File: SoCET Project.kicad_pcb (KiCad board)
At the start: 2 copper layers, 80.5 x 48.7 mm, 45 parts, among them J1 USB_C_Receptacle_USB2.0, J2 Conn_01x16_Female, J3 Conn_01x16_Female, J6 ICSP, SW1 SW_Push, U1 ATmega328P-A, U2 LM1117DT-ADJ, U3 FT232RL, Y1 16MHz

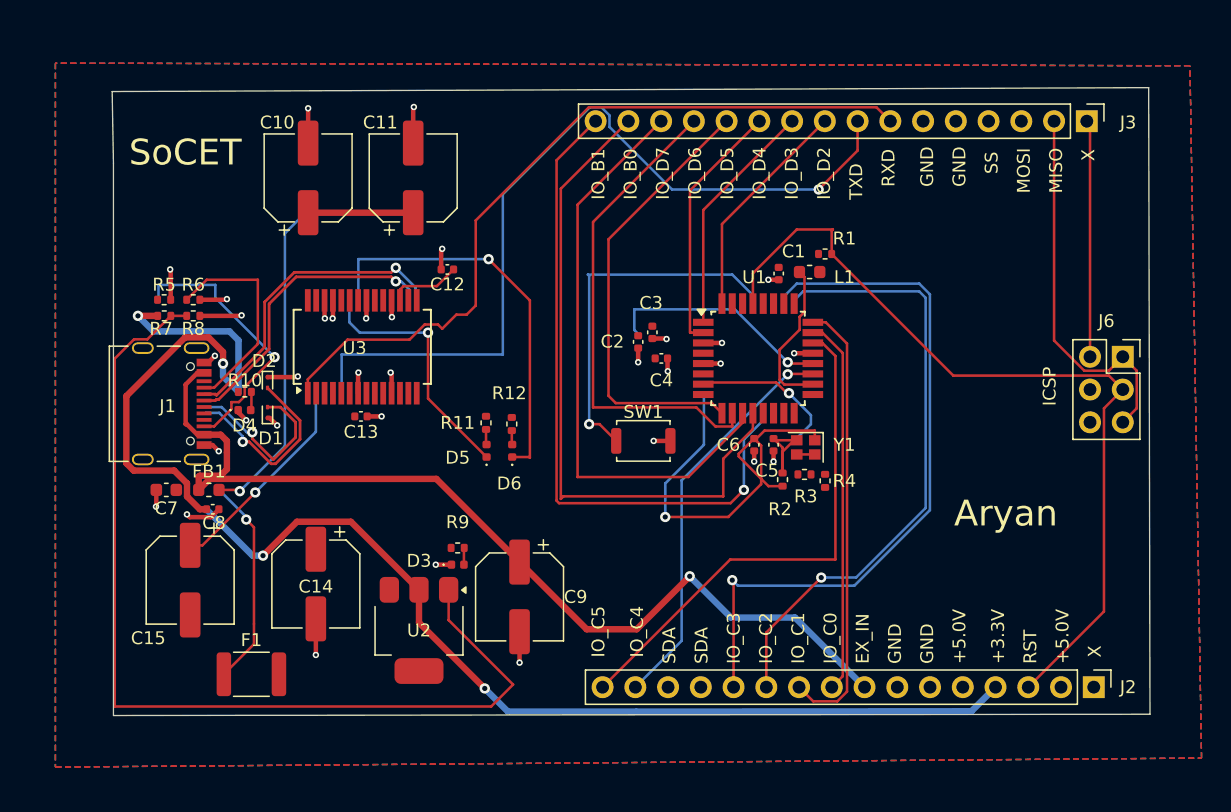
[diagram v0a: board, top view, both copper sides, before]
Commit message: Add files via upload
Completed SCH and DSG
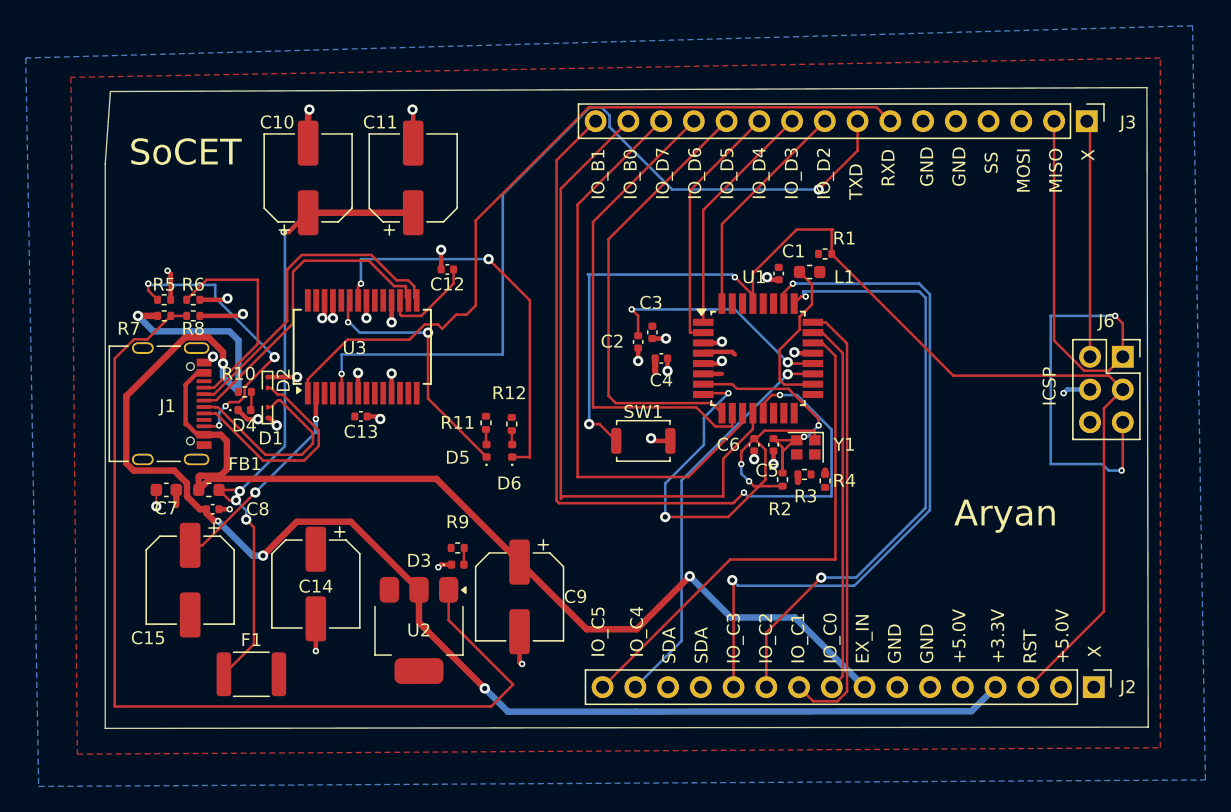
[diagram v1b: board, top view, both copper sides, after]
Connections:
- D1 pad 2: USBC_D.P -> USBC_D.N
- D2 pad 2: USBC_D.N -> USBC_D.P
- U3 pad 15: USBC_D.P -> USBC_D.N
- U3 pad 16: USBC_D.N -> USBC_D.P
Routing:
- net SPI.MISO: track 29.7 -> 53.2 mm, vias 0 -> 2
- net GPIO_B1: track 51.9 -> 65.2 mm, vias 1 -> 2
- net +5V: track 0.00 -> 7.10 mm
- net USBC_D.P: track 36.8 -> 42.2 mm, vias 2 -> 0
- net EX_OSC2: track 34.9 -> 38.6 mm, vias 1 -> 4
- net USBC_D.N: track 39.4 -> 41.4 mm, vias 2 -> 0
- net Net-(U3-3V3OUT): track 5.64 -> 7.42 mm
- net Net-(J1-CC2): track 21.3 -> 23.0 mm, vias 1 -> 4
- net (no net): track 1.40 -> 0.00 mm
- net EX_OSC1: track 19.6 -> 20.9 mm, vias 1 -> 2
- net GND: track 53.4 -> 54.6 mm
- net Net-(C10-Pad1): track 49.8 -> 50.6 mm, vias 2 -> 4
- net EX_RST: track 92.7 -> 93.3 mm, vias 1 -> 2
- net GPIO_C2: track 47.6 -> 48.2 mm, vias 1 -> 2
- net GPIO_C3: track 55.2 -> 55.8 mm, vias 1 -> 2
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- removed copper zone on B.Cu, net +5V
- removed copper zone on F.Cu, net GND
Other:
- board size 80.5 x 48.7 mm -> 80.9 x 49.7 mm
